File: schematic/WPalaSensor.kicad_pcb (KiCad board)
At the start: 2 copper layers, 25.4 x 29.8 mm, 8 parts, among them P3 Palazzetti Connector, U1 WeMos_mini, U3 DS18B20, U4 MCP4151-50k, U5 MCP4151-5k

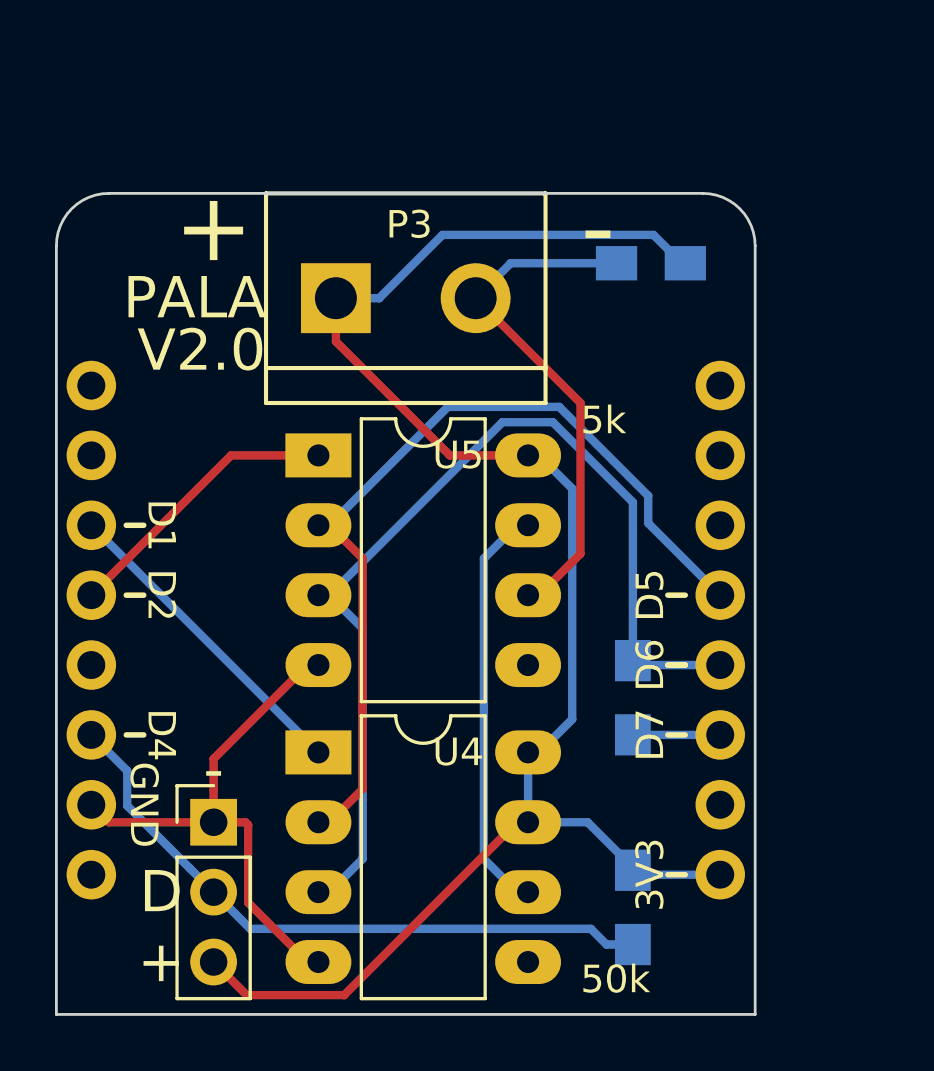
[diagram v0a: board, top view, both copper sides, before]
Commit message: Update schematic
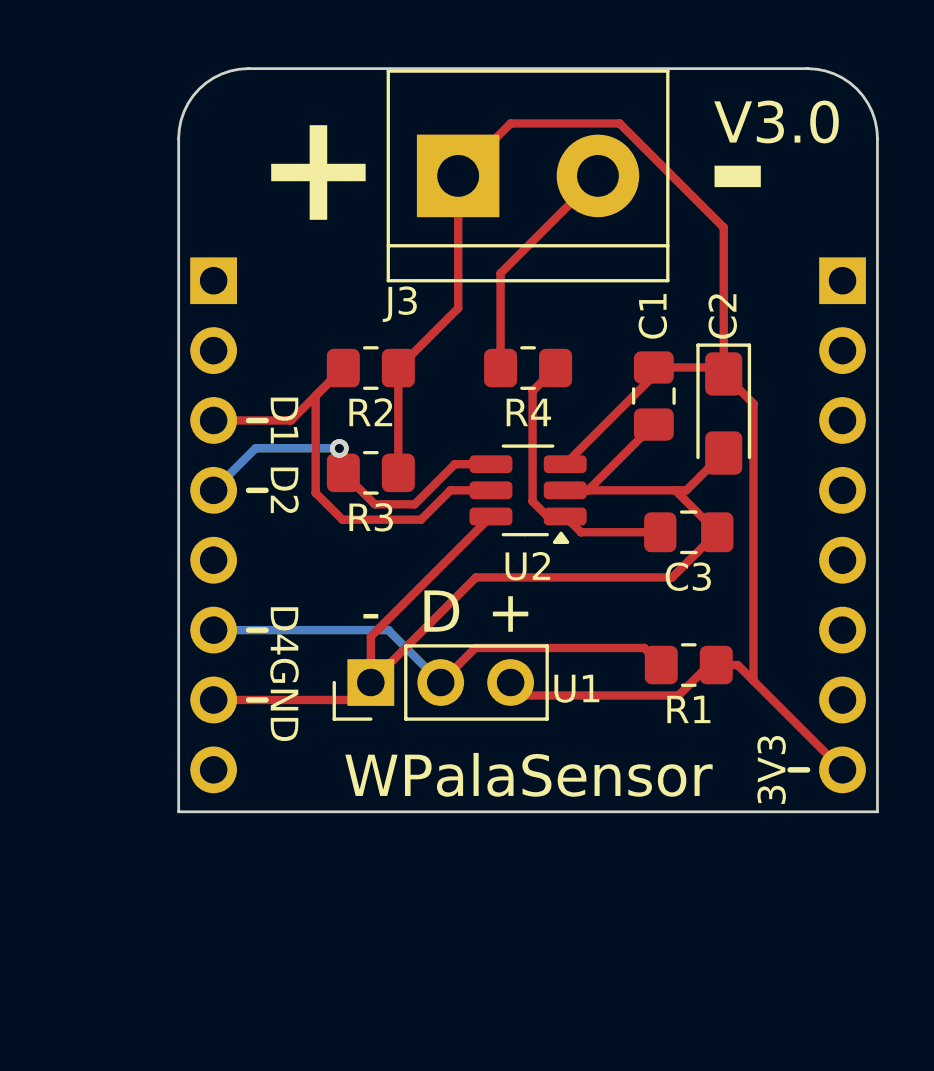
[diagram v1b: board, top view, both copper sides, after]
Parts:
- removed P3: Palazzetti Connector, Connect:bornier2
- removed U3: DS18B20, Pin_Headers:Pin_Header_Straight_1x03_Pitch2.54mm
- removed U4: MCP4151-50k, Housings_DIP:DIP-8_W7.62mm_LongPads
- removed U5: MCP4151-5k, Housings_DIP:DIP-8_W7.62mm_LongPads
- added C1: 100n, Capacitor_SMD:C_0805_2012Metric_Pad1.18x1.45mm_HandSolder, F.Cu at (41.4, 29.6)
- added C2: 10u, Capacitor_Tantalum_SMD:CP_EIA-3216-18_Kemet-A_Pad1.58x1.35mm_HandSolder, F.Cu at (43.9, 30.2)
- added J1: WeMos_mini_Hat_Left, wemos_d1_mini:WeMos_D1_mini_Hat_Left, B.Cu at (25.4, 25.4)
- added J2: WeMos_mini_Hat_Right, wemos_d1_mini:WeMos_D1_mini_Hat_Right, B.Cu at (48.3, 25.4)
- added J3: Fumis T01, TerminalBlock:TerminalBlock_bornier-2_P5.08mm, F.Cu at (34.3, 21.6)
- added R3: 4.7K, Resistor_SMD:R_0805_2012Metric_Pad1.20x1.40mm_HandSolder, F.Cu at (31.1, 32.4)
- added R4: 2.2K 1%, Resistor_SMD:R_0805_2012Metric_Pad1.20x1.40mm_HandSolder, F.Cu at (36.8, 28.6)
- added U2: MCP4725, Package_TO_SOT_SMD:SOT-23-6_Handsoldering, F.Cu at (36.8, 33.0)
- C3: value 1uF -> 100n; footprint Capacitors_SMD:C_0805_HandSoldering -> Capacitor_SMD:C_0805_2012Metric_Pad1.18x1.45mm_HandSolder; moved to F.Cu
- R1, R2: footprint Resistors_SMD:R_0805_HandSoldering -> Resistor_SMD:R_0805_2012Metric_Pad1.20x1.40mm_HandSolder; moved to F.Cu
- U1: value WeMos_mini -> DS18B20; footprint wemos_d1_mini:wemos-d1-mini-DIL-only -> Connector_PinHeader_2.54mm:PinHeader_1x03_P2.54mm_Vertical; moved to F.Cu
- moved R2 15.3 mm to (31.1, 28.6), turned to 180 degrees
- moved C3 9.88 mm to (42.7, 34.5), turned to 0 degrees
- moved R1 9.04 mm to (42.7, 39.4), turned to 180 degrees
- moved U1 2.29 mm to (31.1, 40.0)
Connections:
- C3 pad 1: VCC -> Net-(U2-VOUT)
- C3 pad 2: Net-(C3-Pad2) -> GND
- R1 pad 2: Net-(R1-Pad2) -> Net-(J1-D4)
- R2 pad 1: Net-(R2-Pad1) -> VCC
- R2 pad 2: Net-(R2-Pad2) -> Net-(J1-D1)
- U1 pad 1: (no net) -> GND
- U1 pad 2: GND -> Net-(J1-D4)
- U1 pad 3: Net-(R1-Pad2) -> VCC
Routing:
- net Net-(R2-Pad1): track 36.4 -> 0.00 mm
- net Net-(U1-Pad12): track 32.4 -> 0.00 mm
- net Net-(R1-Pad2): track 23.6 -> 0.00 mm
- net GND: track 19.8 -> 41.4 mm
- net Net-(C3-Pad2): track 19.0 -> 0.00 mm
- net Net-(J1-D4): track 0.00 -> 17.8 mm
- net Net-(J1-D1): track 0.00 -> 17.7 mm
- net Net-(U4-Pad6): track 15.1 -> 0.00 mm
- net Net-(J1-D2): track 0.00 -> 12.6 mm, vias 0 -> 1
- net Net-(U1-Pad6): track 11.7 -> 0.00 mm
- net Net-(U1-Pad5): track 10.4 -> 0.00 mm
- net Net-(U2-VOUT): track 0.00 -> 10.3 mm
- net Net-(J3-Pin_2): track 0.00 -> 8.45 mm
- net Net-(R2-Pad2): track 3.17 -> 0.00 mm
- net VCC: track 61.9 -> 62.4 mm
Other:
- board size 25.4 x 29.8 mm -> 25.4 x 27 mm
- board text added: "C1,C3: 100n C2: 10u R1,R2,R3: 4.7K R4: 2.2K 1% U2: MCP4725"
- board text added: "JLCJLCJLCJLC"
- board text added: "V3.0"
- board text added: "WPalaSensor"
- board text removed: "50k"
- board text removed: "5k"
- board text removed: "D5"
- board text removed: "D6"
- board text removed: "D7"
- board text removed: "PALA"
- board text removed: "V2.0"
- board text removed: "WirelessPalaSensor"
